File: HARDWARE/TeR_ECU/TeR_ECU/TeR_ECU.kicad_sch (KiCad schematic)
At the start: 0 parts

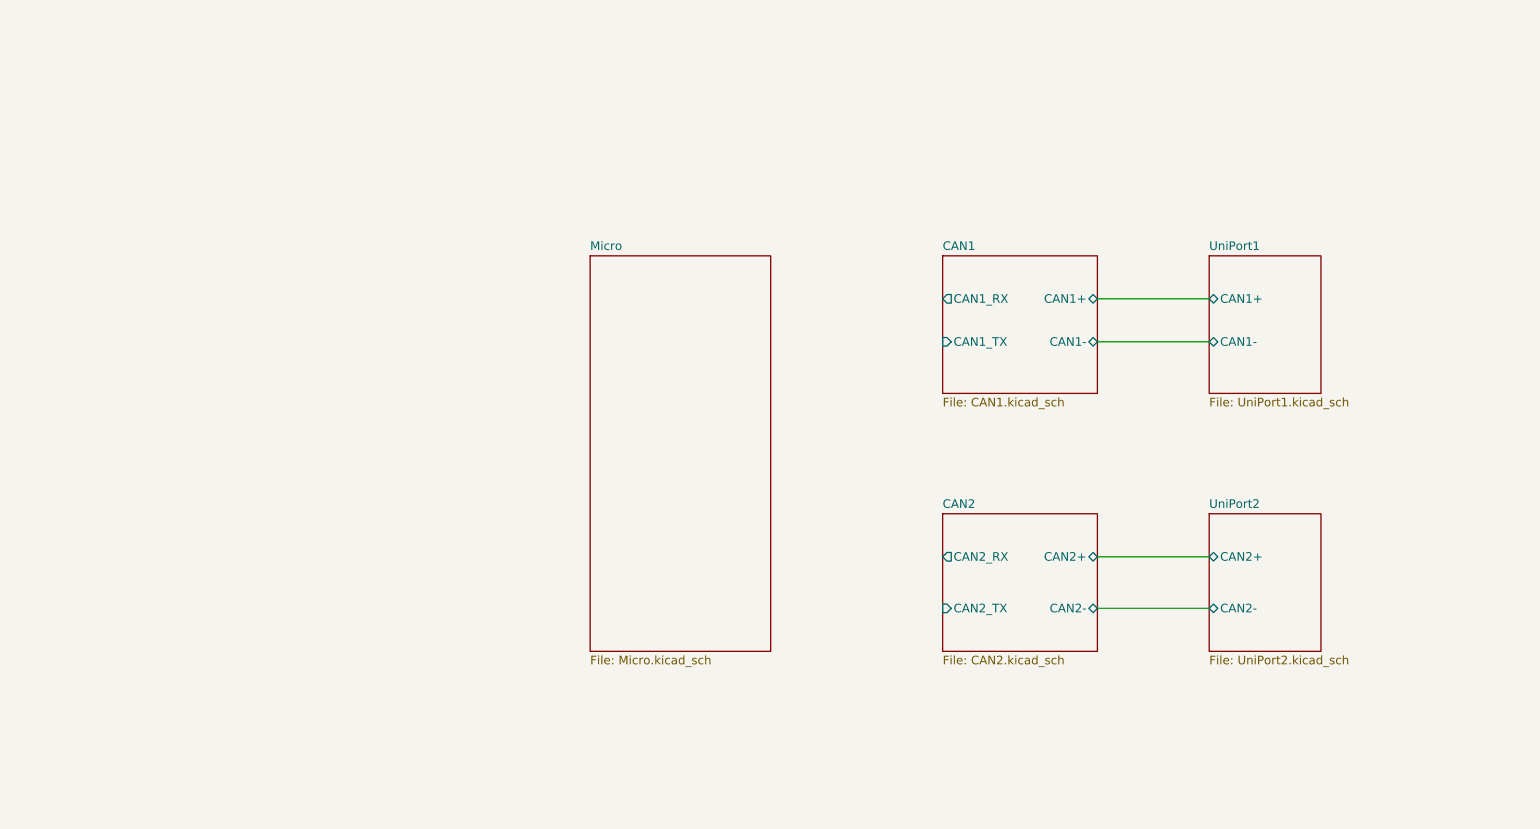
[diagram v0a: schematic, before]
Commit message: Menos el del conector grande, los demas esquematicos acabados
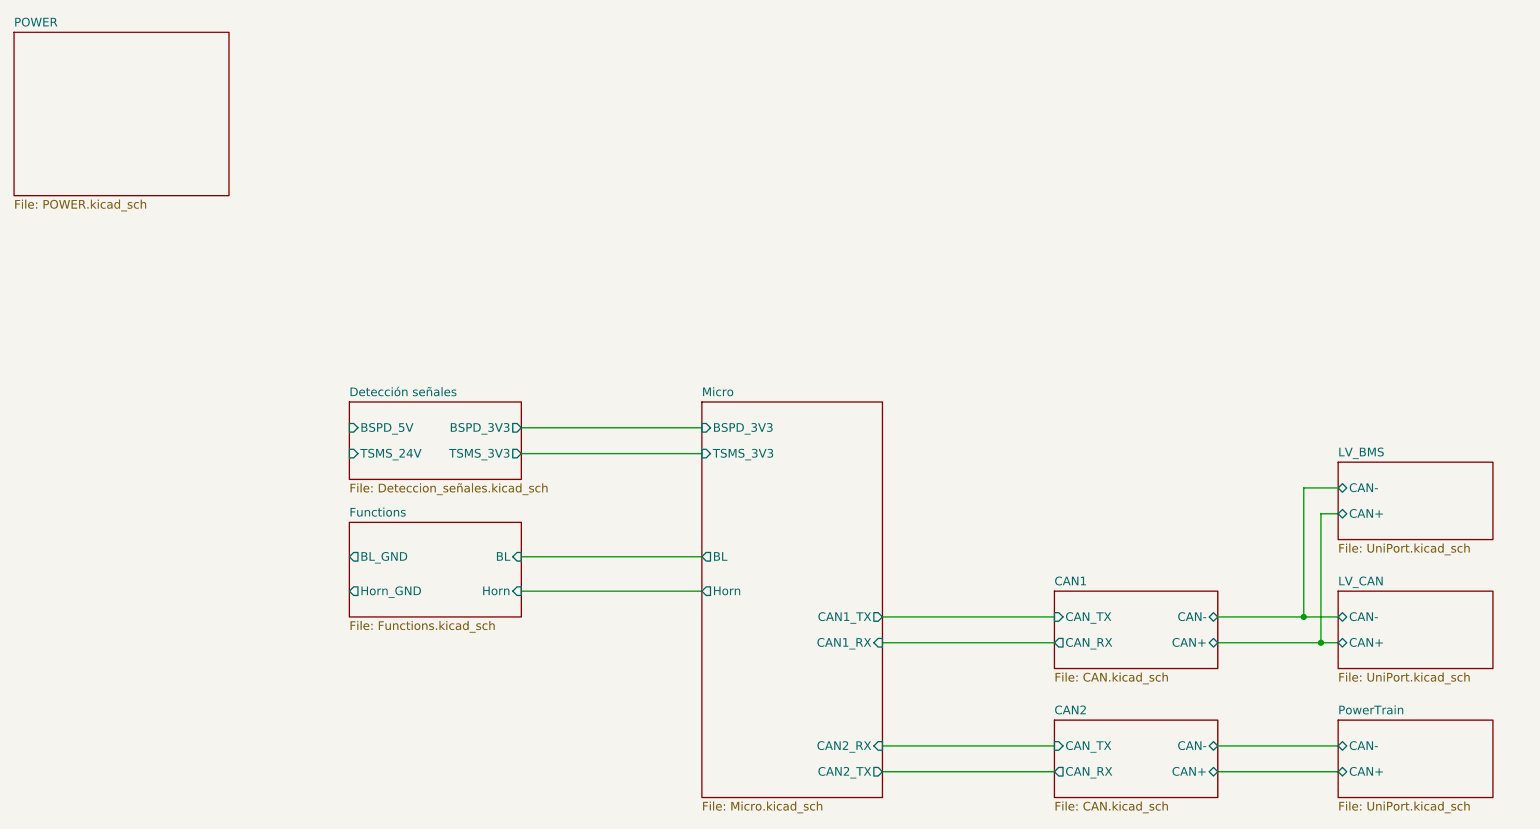
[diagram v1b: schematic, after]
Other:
- removed sheet UniPort1
- removed sheet UniPort2
- added sheet Detección señales (Deteccion_señales.kicad_sch)
- added sheet Functions (Functions.kicad_sch)
- added sheet LV_BMS (UniPort.kicad_sch)
- added sheet LV_CAN (UniPort.kicad_sch)
- added sheet POWER (POWER.kicad_sch)
- added sheet PowerTrain (UniPort.kicad_sch)
- sheet CAN1: file CAN1.kicad_sch -> CAN.kicad_sch
- sheet CAN1 ports: added CAN+, CAN-, CAN_RX, CAN_TX; removed CAN1+, CAN1-, CAN1_RX, CAN1_TX
- sheet CAN2: file CAN2.kicad_sch -> CAN.kicad_sch
- sheet CAN2 ports: added CAN+, CAN-, CAN_RX, CAN_TX; removed CAN2+, CAN2-, CAN2_RX, CAN2_TX
- sheet Micro ports: added BL, BSPD_3V3, CAN1_RX, CAN1_TX, CAN2_RX, CAN2_TX, Horn, TSMS_3V3; removed none
